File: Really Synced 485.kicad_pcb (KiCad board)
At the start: 2 copper layers, 34 parts, among them J1 CONN_02X04, J2 CONN_01X03, J3 CONN_01X03, J4 CONN_02X04, U1 CE_HEADER, U2 SN75179B, U3 SN65HVD82

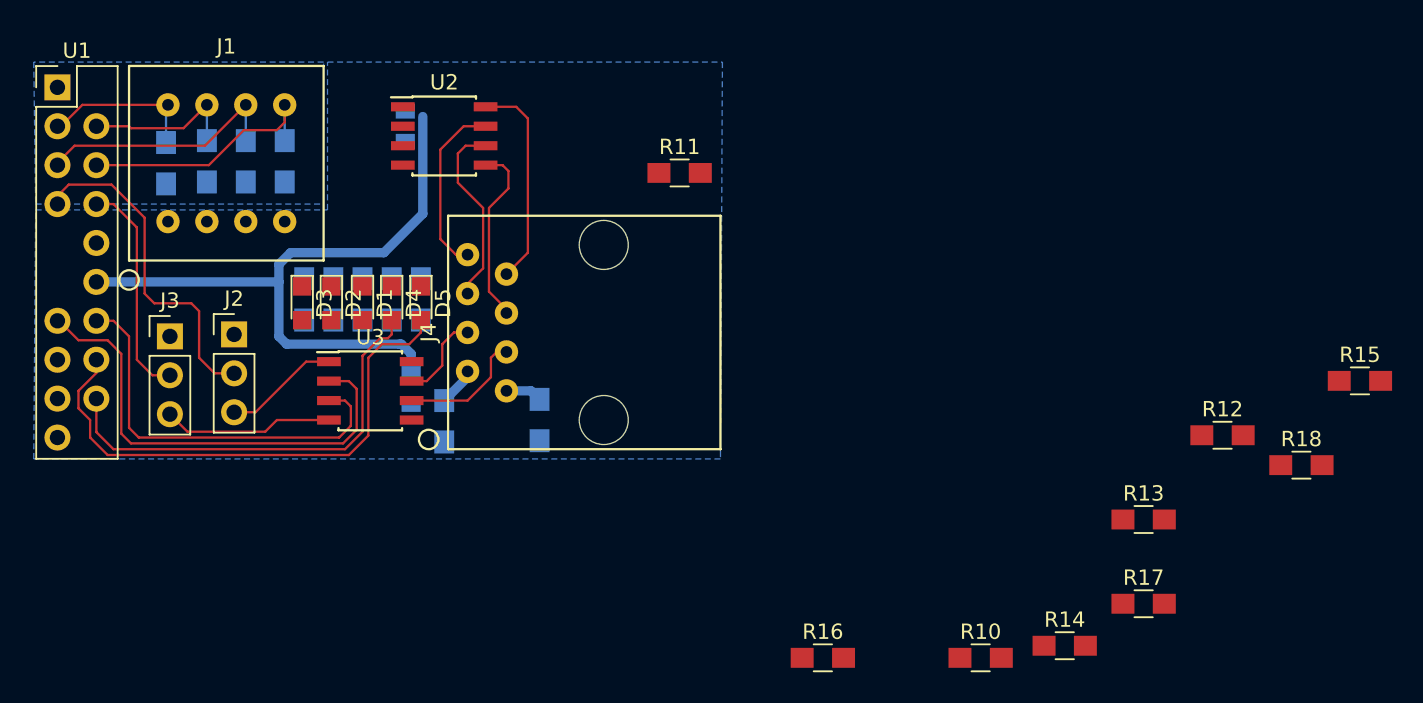
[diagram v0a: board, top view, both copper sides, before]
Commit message: Finished initial layout, doing DRC next
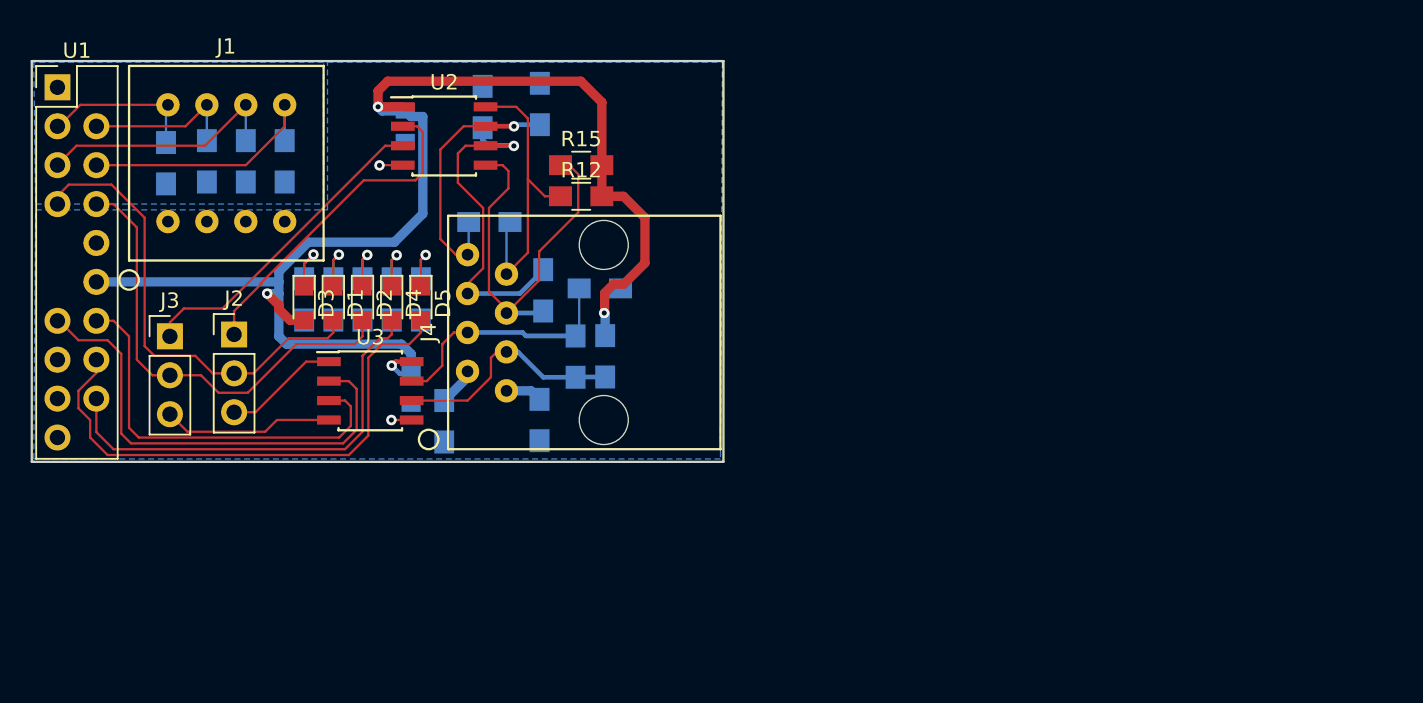
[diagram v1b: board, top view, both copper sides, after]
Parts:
- R10, R11, R13, R14, R16, R17, R18: moved to B.Cu
- moved R15 52.8 mm to (157.3, 109.7)
- moved R14 51.8 mm to (150.8, 105.9), turned to 90 degrees
- moved R13 47.8 mm to (154.6, 105.7), turned to 90 degrees
- moved R18 47.2 mm to (158.5, 117.8)
- moved R12 44.7 mm to (157.3, 111.8)
- moved R10 42.9 mm to (151.3, 113.4)
- moved R17 40.4 mm to (156.9, 122.2), turned to 90 degrees
- moved R16 24.3 mm to (158.8, 122.2), turned to 270 degrees
- moved R11 11.7 mm to (154.8, 117.9), turned to 90 degrees
- moved D2 2.03 mm to (143.0, 118.7)
- moved D1 1.91 mm to (141.1, 118.7)
- moved R1 1.91 mm to (141.1, 118.5)
- moved R4 1.91 mm to (143.0, 118.5)
- moved D3 0.13 mm to (139.2, 118.7)
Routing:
- net +5V: track 44.0 -> 90.7 mm, vias 0 -> 4
- net /RX_FULL: track 0.00 -> 21.8 mm
- net /TX_FULL: track 0.00 -> 20.9 mm
- net /TX: track 14.5 -> 30.1 mm
- net /Y: track 11.9 -> 27.4 mm
- net /Z: track 12.3 -> 22.7 mm, vias 0 -> 1
- net /B_HALF: track 5.78 -> 16.1 mm
- net /RX: track 22.2 -> 30.8 mm
- net /A_HALF: track 8.76 -> 15.9 mm
- net /A: track 13.8 -> 19.9 mm
- net /B: track 11.6 -> 17.4 mm, vias 0 -> 1
- net Net-(D3-Pad1): track 0.00 -> 4.17 mm, vias 0 -> 1
- net Net-(D1-Pad1): track 0.00 -> 3.94 mm, vias 0 -> 1
- net Net-(D5-Pad1): track 0.00 -> 3.87 mm, vias 0 -> 1
- net Net-(D2-Pad1): track 0.00 -> 3.86 mm, vias 0 -> 1
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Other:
- board outline added: 45.1 x 26.2 mm
